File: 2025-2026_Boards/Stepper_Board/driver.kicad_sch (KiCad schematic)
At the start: 1 part

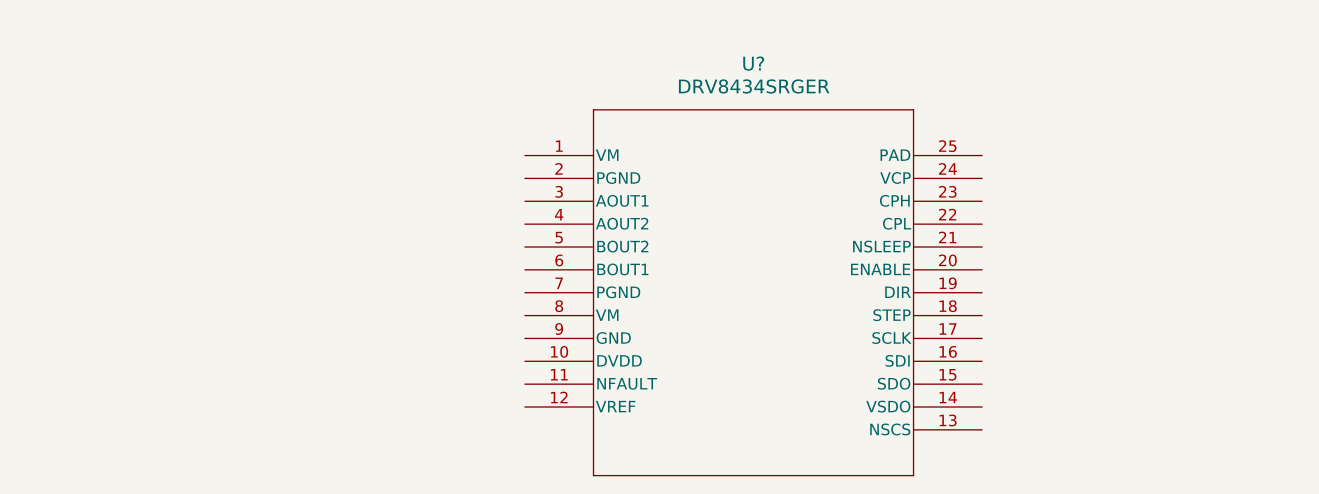
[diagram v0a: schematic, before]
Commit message: finished driver
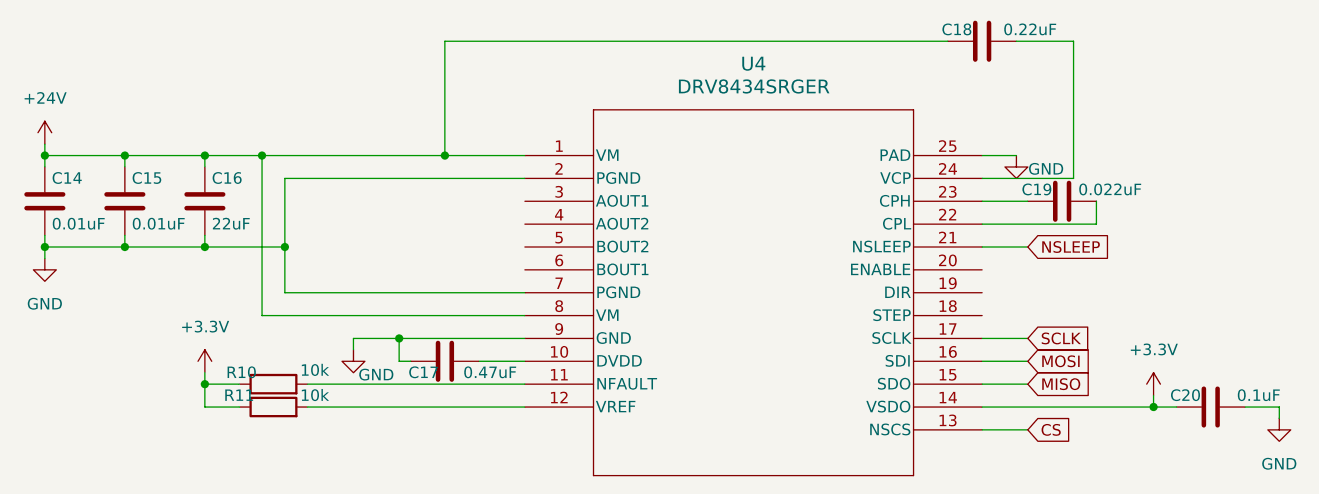
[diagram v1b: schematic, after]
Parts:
- added C14, C15: 0.01uF, symbol Device:C
- added C16: 22uF, symbol Device:C
- added C17: 0.47uF, symbol Device:C
- added C18: 0.22uF, symbol Device:C
- added C19: 0.022uF, symbol Device:C
- added C20: 0.1uF, symbol Device:C
- added R10, R11: 10k, symbol Device:R
- gave numbers to parts that had none: 1
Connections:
- net +24V: now reaches U4.1 (VM)
- net +24V: now also U4.8 (VM), C14.1, C15.1, C16.1, C18.1
- net at U4.10 (DVDD): now also C17.1
- net at U4.11 (NFAULT): now also R10.2
- net at U4.12 (VREF): now also R11.2
- net CS: now reaches U4.13 (NSCS)
- net +3.3V: now reaches U4.14 (VSDO)
- net +3.3V: now also C20.1, R10.1, R11.1
- net MISO: now reaches U4.15 (SDO)
- net MOSI: now reaches U4.16 (SDI)
- net SCLK: now reaches U4.17 (SCLK)
- net GND: now reaches U4.2 (PGND)
- net GND: now also U4.25 (PAD), U4.7 (PGND), U4.9 (GND), C14.2, C15.2, C16.2, C17.2, C20.2
- net NSLEEP: now reaches U4.21 (NSLEEP)
- net at U4.22 (CPL): now also C19.2
- net at U4.23 (CPH): now also C19.1
- net at U4.24 (VCP): now also C18.2
